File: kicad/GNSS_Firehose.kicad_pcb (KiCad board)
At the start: 4 copper layers, 117.9 x 99.1 mm, 460 parts, among them J1 SMA, J10 HEADER_16, J2 SMA, J3 SMA, J4 SMA, J5 SMA, J6 HEADER_14, J7 L829-1J1T-43, J8 PJ-063BH, Q1 Si2369DS, U1 MAX2112, U10 MAX19505, U11 AT25DF041A, U12 XC6SLX9-2TQG144C, U15 LMK03806, U17 LTC3633, U18 KSZ9031RNX, U19 CDCLVC1102, U2 MAX19505, U20 MIC2090-1YM5, U21 MIC2090-1YM5, U22 MIC2090-1YM5, U3 MGA-68563, U4 MAX2112, U5 MAX19505, U6 MGA-68563, U7 MAX2112, U8 MAX19505, U9 MGA-68563, Y1 25 MHz

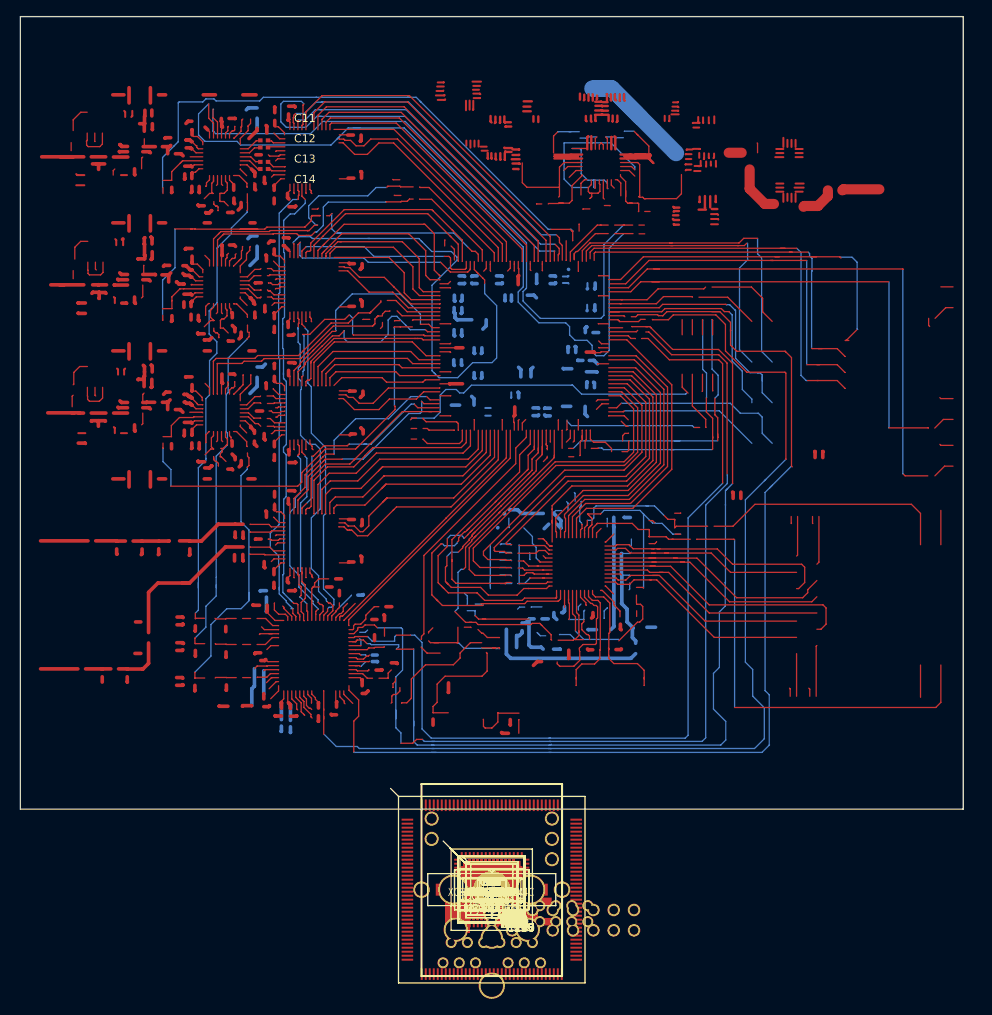
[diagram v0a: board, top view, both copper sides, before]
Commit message: initial placement and wires
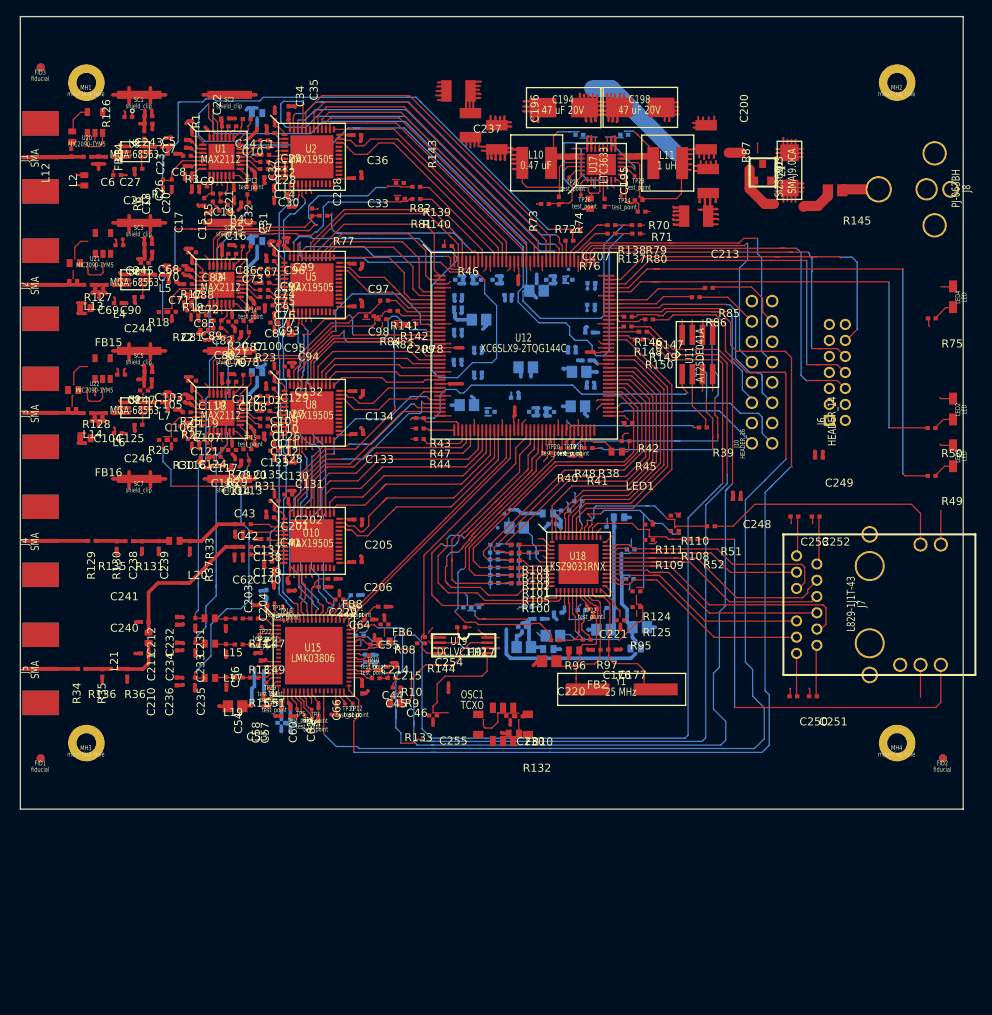
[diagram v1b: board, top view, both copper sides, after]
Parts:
- C141, C142, C143, C144, C145, C146, C147, C148, C149, C150, C151, C152, C153, C154, C155, C156, C157, C158, C159, C160, C161, C162, C163, C164, C165, C166, C167, C168, C182, C183, C184, C185, C186, C187, C193, C197, C199, C216, C217, C218, C219, C222, C223, C224, C225, C226, C227, C228, C59, C63, C65, FB1, FB11, FB12, FB13, FB3, FB4, FB5, FB7, FB9, R106, R107, R112, R113, R114, R115, R116, R117, R118, R119, R120, R121, R122, R123, R98, R99: moved to B.Cu
- moved FID3 117.2 mm to (76.2, 49.5)
- moved MH1 112.9 mm to (81.9, 51.4)
- moved MH2 112.9 mm to (183.3, 51.4)
- moved J1 109.1 mm to (73.2, 60.8), turned to 90 degrees
- moved SC1 108.7 mm to (88.5, 53.0)
- moved R126 107.8 mm to (80.1, 58.2), turned to 90 degrees
- moved U20 107.3 mm to (82.0, 57.7)
- moved C243 106.7 mm to (87.1, 55.7)
- moved J8 106.3 mm to (192.9, 64.8), turned to 270 degrees
- moved L12 106.1 mm to (80.0, 60.2), turned to 270 degrees
- moved C5 105.8 mm to (89.7, 55.6)
- moved C7 104.9 mm to (89.7, 56.6)
- moved C6 104.6 mm to (82.0, 60.7)
- moved SC2 104.6 mm to (99.8, 53.0)
- moved L3 103.9 mm to (89.2, 58.0), turned to 270 degrees
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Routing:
- net (no net): track 6403.4 -> 2297.0 mm
- net GND: track 0.00 -> 357.5 mm, vias 0 -> 1
- net VCC_3.3V: track 0.00 -> 235.2 mm
- net /Ethernet/DVDDL: track 0.00 -> 50.6 mm
- net PHY_RXD3: track 0.00 -> 46.7 mm
- net CH1_CLK: track 0.00 -> 44.0 mm
- net PHY_RX_CTL: track 0.00 -> 43.0 mm
- net PHY_RXD0: track 0.00 -> 42.3 mm
- net CH1_D7: track 0.00 -> 41.5 mm
- net PHY_RXD1: track 0.00 -> 40.1 mm
- net CH1_D6: track 0.00 -> 39.3 mm
- net VCC_1.2V: track 0.00 -> 38.7 mm
- net PHY_RXD2: track 0.00 -> 38.6 mm
- net CH1_D5: track 0.00 -> 37.1 mm
- net Net-(TP22-Pad1): track 0.00 -> 36.7 mm
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- added copper zone on In1.Cu, net GND
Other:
- net class Default: clearance 0.2 -> 0.1524; trace_width 0.25 -> 0.1524; via_dia 0.6 -> 0.6096; via_drill 0.4 -> 0.3048
- net class wide added: clearance 0.1524, trace_width 0.4572, via_dia 0.6096, via_drill 0.3048
- rule pad_to_mask_clearance: 0.2 -> 0
- rule trace_clearance: 0.2 -> 0.1524
- rule trace_min: 0.2 -> 0.1524
- rule via_min_drill: 0.3 -> 0.3048
- rule via_min_size: 0.4 -> 0.6096
